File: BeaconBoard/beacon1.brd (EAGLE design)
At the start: 113 x 112.7 mm, 108 parts, among them IC1 NCP1117ST50T3G, IC6 LP2985-33DBVR, IC7 LMV358IDGKR, SW1 EG1319, T1 FDN340P, U1 FGPMMOPA6H, U2 MIC5225-3.3, U4 MIC5225-3.3, U5 MB85RC256VPF-G-JNERE2, X1 JST 2PH, Y1 CSTCE16M0V53-R0 16MHZ, Y2 32.768kHz (535-9166-2-ND)

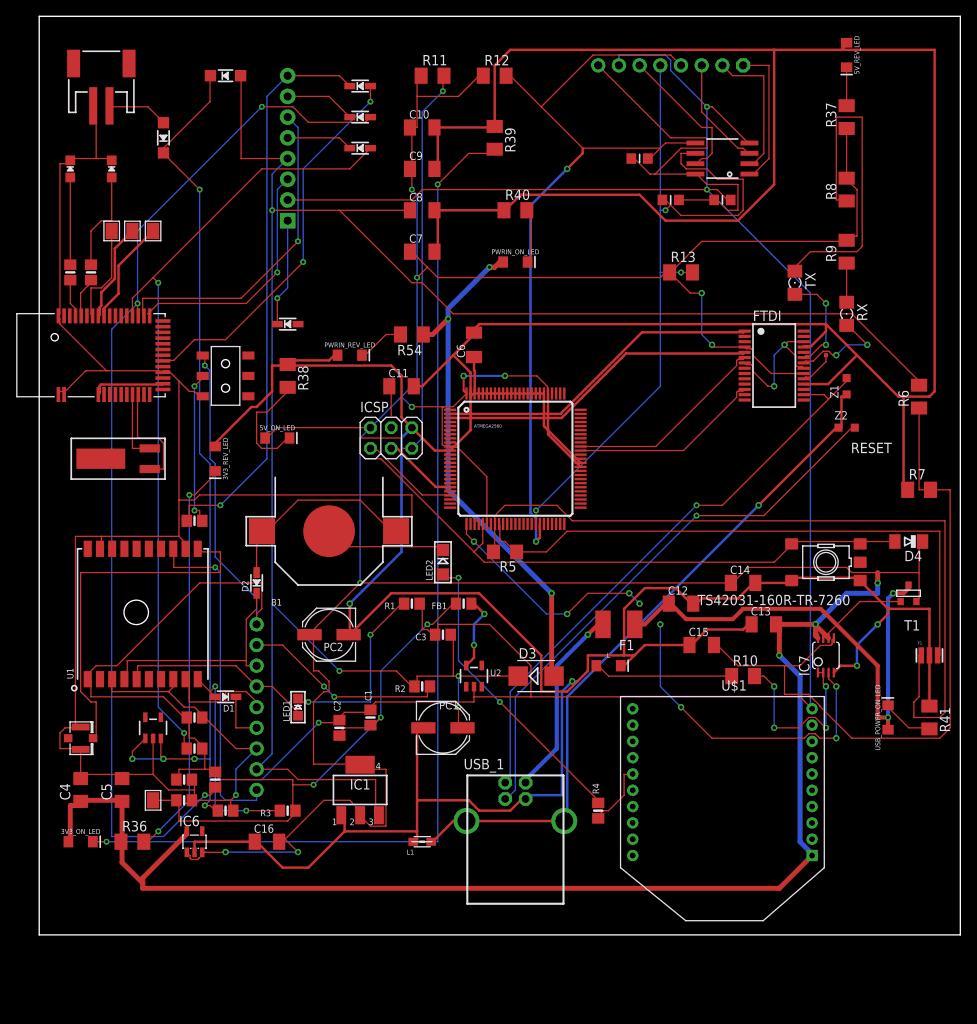
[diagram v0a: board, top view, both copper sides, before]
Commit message: i changed everything and only just comitted now cause im bad
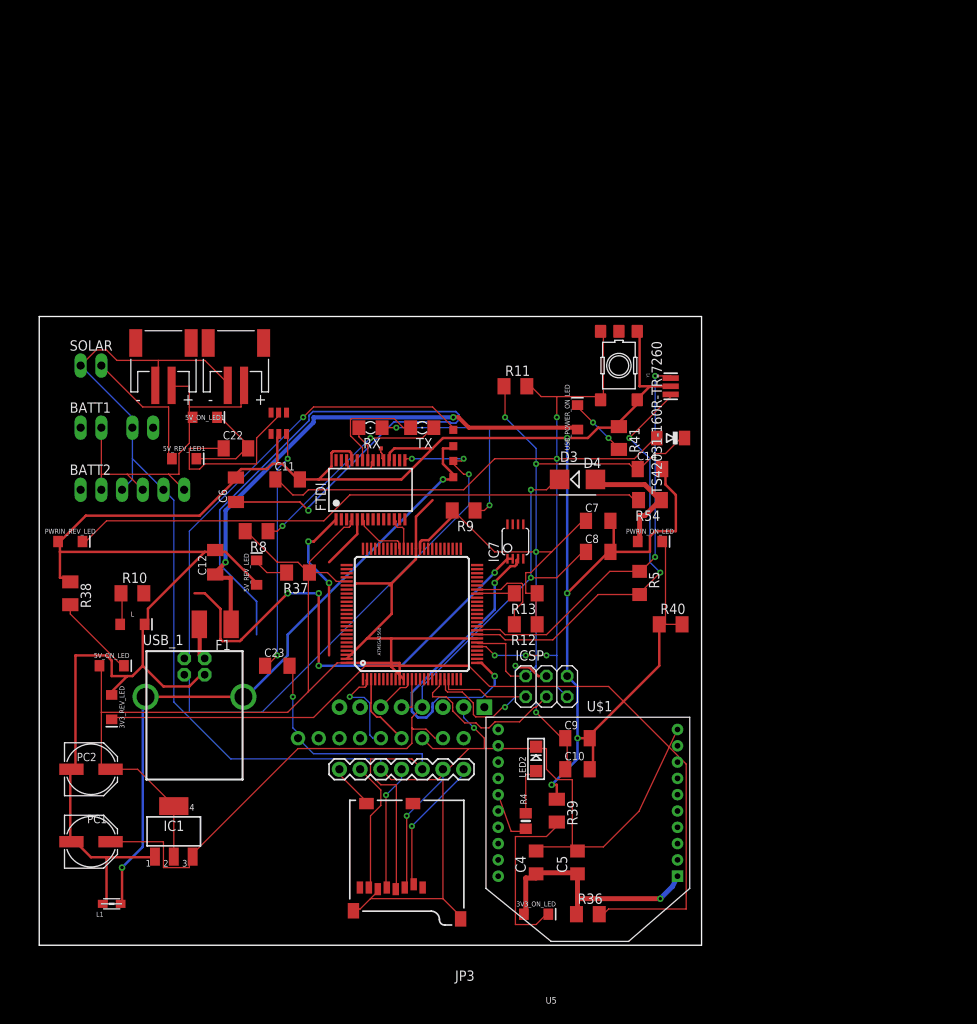
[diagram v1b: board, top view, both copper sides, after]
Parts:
- removed B1: CR1220, microbuilder:CR1220
- removed C1: 0.1uF, microbuilder:0805-NO
- removed C13: 1u, SmartPrj:C1206K
- removed C15, C16: 100n, SmartPrj:C1206K
- removed C17, C18: 1uF, microbuilder:0805-NO
- removed C19, C2, C20, C3: 10uF, microbuilder:0805-NO
- removed C21: 10uF, microbuilder:_0805MP
- removed D1: 1N4148, microbuilder:SOD-323
- removed D10, D11, D8, D9: 1n4148, microbuilder:SOD-323
- removed D12, D7: MBR120, microbuilder:SOD-123
- removed D2: CUS520, microbuilder:SOD-323
- removed D5: RED, microbuilder:CHIPLED_0805_NOOUTLINE
- removed D6: GREEN, microbuilder:CHIPLED_0805_NOOUTLINE
- removed FB1: Ferrite, microbuilder:0805-NO@1
- removed IC6: LP2985-33DBVR, SmartPrj:SOT23-DBV
- removed LED1: RED, microbuilder:CHIPLED_0805
- removed R1, R14, R15: 1K, microbuilder:0805-NO
- removed R16, R17: 100K, microbuilder:0805-NO
- removed R18: 2K, microbuilder:0805-NO
- removed R19, R20: 10K, microbuilder:_0805MP
- removed R2, R3: 10K, microbuilder:0805-NO
- removed R6, R7: 10k, adafruit:M1206
- removed SW1: EG1319, microbuilder:EG1390
- removed T1: FDN340P, zetex:SOT-23
- removed TP1: SWCLK, microbuilder:PAD-1.5X2.0
- removed TP2: SWDIO, microbuilder:PAD-1.5X2.0
- removed TP3, VTREF: FCTRST, microbuilder:PAD-1.5X2.0
- removed U$20: U.FL, microbuilder:U.FL
- removed U1: FGPMMOPA6H, microbuilder:FGPMMOPA6H
- removed U2, U4: MIC5225-3.3, microbuilder:SOT23-5
- removed U3: (no value), microbuilder:BLE_MODULE_RAYTAC_MDBT40
- removed X1: JST 2PH, microbuilder:JSTPH2
- removed Y2: 32.768kHz (535-9166-2-ND), microbuilder:CRYSTAL_CYL_2X6MM_SMT
- added 5V_ON_LED1: GREEN, SparkFun-LED:LED-1206
- added 5V_REV_LED1: RED, SparkFun-LED:LED-1206
- added BATT1, BATT2: Battery, microbuilder:1X02_OVAL
- added C22, C23: 100m, SmartPrj:C1206K
- added CN1: BATT_IN_JST, microbuilder:JSTPH2
- added CN4: LOAD_JST, microbuilder:JSTPH2
- added JP10: LOAD_0.1, microbuilder:1X02_OVAL
- added JP11: BATT_IN_0.1, microbuilder:1X02_OVAL
- added JP8: PWR_IN_0.1, microbuilder:1X02_OVAL
- added SOLAR: Solar, microbuilder:1X02_OVAL
- added U$31: DC877A, DC877A:DC877A
- JP3: device microbuilder:1X08_ROUND_70 -> SparkFun:1X07
- U5: value MB85RC256VPF-G-JNERE2 -> microSD; device microbuilder:SOIC8_208MIL -> SparkFun:MICRO-SD-SOCKET-PP
- moved 5V_REV_LED 96.3 mm to (26.7, 44.5), turned to 90 degrees
- moved U5 91.1 mm to (38.1, 16.5), turned to 180 degrees
- moved JP3 90.0 mm to (52.1, 20.3)
- moved R37 87.5 mm to (31.8, 44.5), turned to 180 degrees
- moved R8 83.6 mm to (26.7, 49.5), turned to 180 degrees
- moved R39 82.9 mm to (63.5, 15.2)
- moved C10 81.0 mm to (66.0, 20.3)
- moved R10 75.6 mm to (11.4, 41.9)
- moved C9 72.4 mm to (66.0, 24.1)
- moved JP2 70.3 mm to (45.7, 27.9), turned to 180 degrees
- moved R12 67.4 mm to (59.7, 38.1), turned to 180 degrees
- moved RX 60.1 mm to (40.6, 62.2), turned to 180 degrees
- moved L 58.6 mm to (11.4, 38.1)
- moved C12 57.4 mm to (21.6, 45.7), turned to 90 degrees
- moved R9 56.7 mm to (52.1, 52.1), turned to 180 degrees
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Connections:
- net WP renamed DO
- removed net A0: JP3.1, U5.1
- removed net A1: JP3.2, U5.2
- removed net A2: JP3.3, U5.3
- removed net CMP: C15.2, IC7.5, R6.1, R7.2
- removed net CONNECTED_LED: R15.1, U3.39
- removed net CTS_3V: D8.A, R16.1, U3.28
- removed net DCC: U3.15
- removed net DEC2: U3.41
- removed net DFU_3V: D11.A, U3.24
- removed net FCTRYRST_3V: TP3.P$1, U3.34
- removed net GATE_CMD: IC7.7, T1.3
- removed net MODE_3V: D10.A, U3.18
- removed net MODE_LED: R14.1, U3.38
- removed net N$1: B1.+$1, B1.+$2, D2.A
- removed net N$15: D5.A, R14.2
- removed net N$16: D6.A, R15.2
- removed net N$17: U3.9, Y2.1
- removed net N$18: U3.10, Y2.2
- removed net N$19: R18.2, SW1.P2
- removed net N$2: LED1.C, R1.2
- removed net N$21: C19.1, D12.C, D7.C, U4.1, U4.3
- removed net N$3: FB1.1, U2.5
- removed net N$4: U$20.P$3, U1.P$11
- removed net RX: D1.C, JP1.4
- removed net RXD2: ATMEGA2560.12
- removed net RXD_3V: D9.A, R17.1, U3.29
- removed net RX_3V: D1.A, R3.2, U1.P$10
- removed net SWCLK: TP1.P$1, U3.36
- removed net SWDIO/RST_3V: TP2.P$1, U3.35
- removed net TX: JP1.5, U1.P$9
- removed net TXD2: ATMEGA2560.13
- removed net VBAT: D7.A, X1.2
- removed net VCC: C21.1, JP3.8, R19.2, R20.2, U5.8
- new net +5V: 5V_REV_LED1.A, SOLAR.2
- new net +5V2: 5V_ON_LED1.A, BATT1.2, BATT2.2, CN1.2, CN4.2, JP10.2, JP11.2
- new net 5.0V: JP8.2
- new net CD1: JP3.7, U5.CD2
- new net CS: JP3.1, U5.2
- new net DI: JP3.2, U5.3
- new net GND2: BATT1.1
- new net GND3: BATT2.1
- new net N$22: C23.1, U$31.3
- new net N$23: C22.1, U$31.5
- new net N$26: 5V_ON_LED1.C, 5V_REV_LED1.C, C22.2
- new net SCK1: JP3.4, U5.5
- new net V+: IC7.8
- new net V-: IC7.4
- net 1PPS: no longer U1.P$13
- net 3.3V: now also C23.2, JP3.3, U5.4; no longer C1.1, C17.1, C18.1, C2.1, C20.1, FB1.2, R16.2, R17.2, R3.1, SW1.O2, U1.P$1, U3.14, U3.3, U4.5, VTREF.P$1
- net 3V3: no longer C13.2, IC6.5, IC7.6
- net 5V: no longer C16.2, IC6.1, IC6.3, IC7.8, T1.2
- net 90348: now also U$31.2; no longer C13.1, C15.1, C16.1, IC6.2, IC7.4, R7.1
- net CTS_5V: no longer D8.C
- net DFU_5V: no longer D11.C
- net ENABLE: no longer R2.1, U2.3
- net FIX: no longer LED1.A, U1.P$5
- net GND: now also CN1.1, CN4.1, JP10.1, JP11.1, JP3.5, JP8.1, SOLAR.1, U5.6, U5.GND1, U5.GND2; no longer B1.-, C1.2, C17.2, C18.2, C19.2, C2.2, C20.2, C21.2, C3.2, D5.C, D6.C, JP3.7, R1.1, SW1.S2, U$20.P$1, U$20.P$2, U1.P$12, U1.P$19, U1.P$3, U1.P$8, U2.2, U3.1, U3.13, U3.16, U3.2, U3.25, U3.42, U4.2, U5.4, X1.1
- net MODE_5V: no longer D10.C, R18.1
- net RTS_O: no longer U3.26
- net RXD0: now also JP1.5
- net RXD_5V: now also ATMEGA2560.13; no longer D9.C
- net SCL: no longer JP3.5, R19.1, U5.6
- net SDA: no longer JP3.4, R20.1, U5.5
- net TXD0: now also JP1.4
- net TX_O: now also ATMEGA2560.12; no longer U3.27
- net USBVCC: no longer T1.1
- net VBACKUP: no longer D2.C, U1.P$4
- net VIN: no longer C3.1, D12.A, R2.2, R6.2, U2.1
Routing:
- net GND: track 504.1 -> 212.4 mm, vias 4 -> 1
- net 90348: track 614.1 -> 374.3 mm
- net 5V: track 409.6 -> 231.6 mm, vias 12 -> 4
- net VIN: track 257.2 -> 100.9 mm, vias 4 -> 2
- net CTS_3V: track 128.5 -> 0.00 mm, vias 3 -> 0
- net 3.3V: track 181.2 -> 52.8 mm, vias 4 -> 1
- net 3V3: track 153.2 -> 30.5 mm
- net N$21: track 111.8 -> 0.00 mm, vias 5 -> 0
- net N$120: track 132.0 -> 21.5 mm, vias 2 -> 0
- net RXD_3V: track 98.7 -> 0.00 mm, vias 2 -> 0
- net SDA: track 103.1 -> 11.3 mm, vias 2 -> 0
- net SCL: track 94.3 -> 4.57 mm, vias 3 -> 0
- net CMP: track 87.1 -> 0.00 mm
- net AREF: track 4.51 -> 85.5 mm, vias 0 -> 1
- net MODE_5V: track 70.3 -> 0.00 mm, vias 1 -> 0
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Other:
- board size 113 x 112.7 mm -> 81.3 x 77.1 mm
